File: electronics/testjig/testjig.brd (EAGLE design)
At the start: 27.4 x 22.9 mm, 13 parts, among them J3 ISP/DUT, Q1 12MHz, U1 MCP1824, U2 TINY84

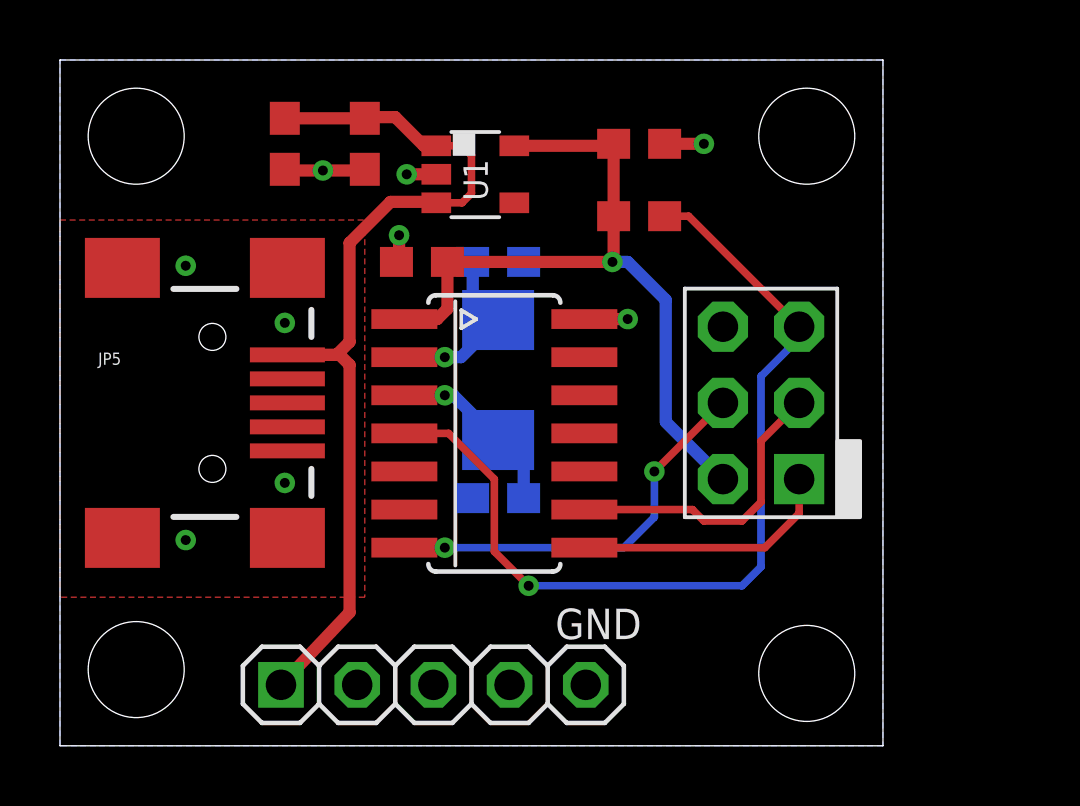
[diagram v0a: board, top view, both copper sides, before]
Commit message: Test jig initial(?)
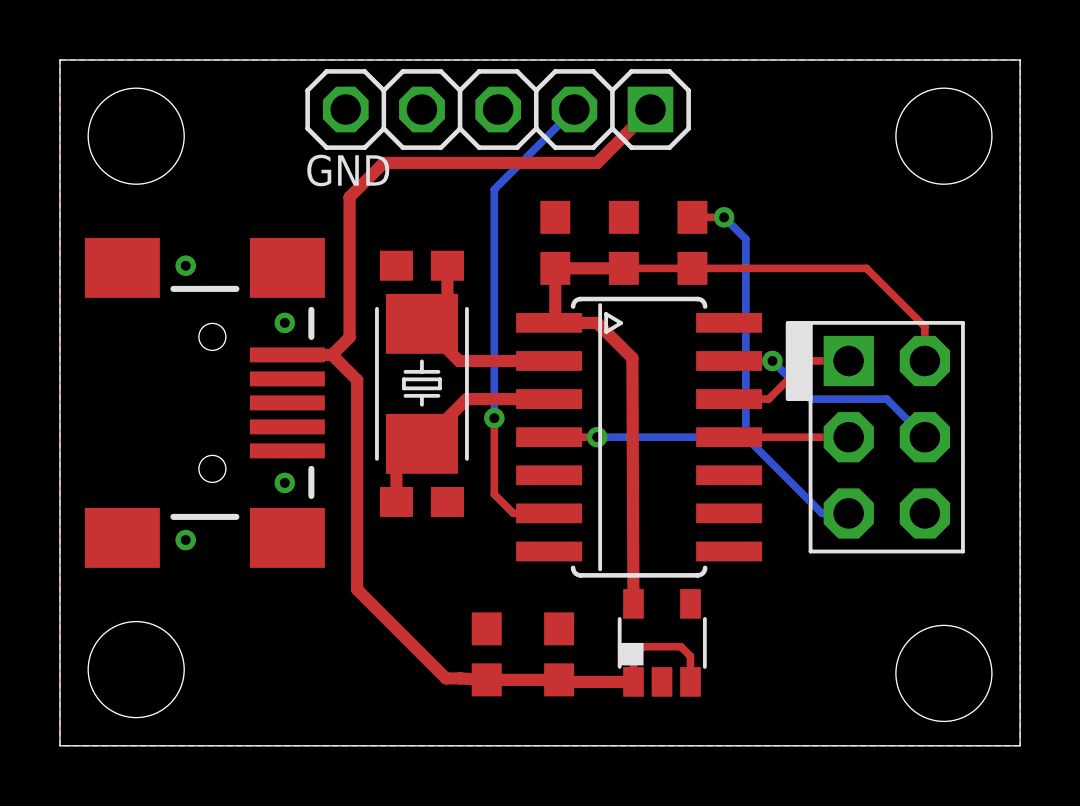
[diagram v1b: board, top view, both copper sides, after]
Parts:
- removed U2: TINY84, bt_avr:SOIC14N
- added IC1: TINY841, bt_avr:SOIC14N
- moved JP4 19.3 mm to (14.6, 21.2), turned to 180 degrees
- moved C4 18.3 mm to (14.2, 3.05), turned to 90 degrees
- moved C3 18.2 mm to (16.6, 3.05), turned to 90 degrees
- moved U1 16.8 mm to (20.1, 3.43), turned to 0 degrees
- moved C1 4.49 mm to (16.5, 16.8), turned to 90 degrees
- moved J3 4.34 mm to (27.6, 10.3), turned to 270 degrees
- moved C2 3.34 mm to (18.8, 16.8), turned to 90 degrees
- moved C5 2.54 mm to (12.1, 8.13), flipped to the top
- moved C6 2.54 mm to (12.1, 16.0), flipped to the top
- moved Q1 2.54 mm to (12.1, 12.1), flipped to the top
- moved R1 1.99 mm to (21.1, 16.8), turned to 270 degrees
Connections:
- removed net N$3: J3.4, U2.7
- removed net N$4: J3.1, U2.8
- removed net N$5: J3.3, U2.9
- new net PA0: IC1.13, J3.4
- new net PA1: IC1.12, J3.1
- new net PA2: IC1.11, J3.3
- net 3.3V: now also IC1.1; no longer U2.1
- net DATA: now also IC1.6
- net GND: now also IC1.14; no longer U2.14
- net RESET: now also IC1.4; no longer U2.4
- net X1: now also IC1.2; no longer U2.2
- net X2: now also IC1.3; no longer U2.3
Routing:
- net DATA: track 0.00 -> 16.0 mm, vias 0 -> 1
- net N$3: track 13.5 -> 0.00 mm, vias 2 -> 0
- net RESET: track 30.2 -> 19.7 mm, vias 1 -> 2
- net N$5: track 10.1 -> 0.00 mm
- net N$4: track 8.78 -> 0.00 mm
- net VBUS: track 32.2 -> 40.8 mm
- net PA0: track 0.00 -> 7.58 mm, vias 0 -> 1
- net GND: track 7.36 -> 0.00 mm, vias 9 -> 4
- net PA1: track 0.00 -> 4.51 mm
- net PA2: track 0.00 -> 3.99 mm
- net 3.3V: track 25.0 -> 27.8 mm, vias 1 -> 0
- net X2: track 6.03 -> 7.15 mm, vias 1 -> 0
- net X1: track 5.93 -> 7.04 mm, vias 1 -> 0
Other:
- board size 27.4 x 22.9 mm -> 32 x 22.9 mm
